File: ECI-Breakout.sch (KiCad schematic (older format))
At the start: 4 parts, among them P1 CONN_02X07

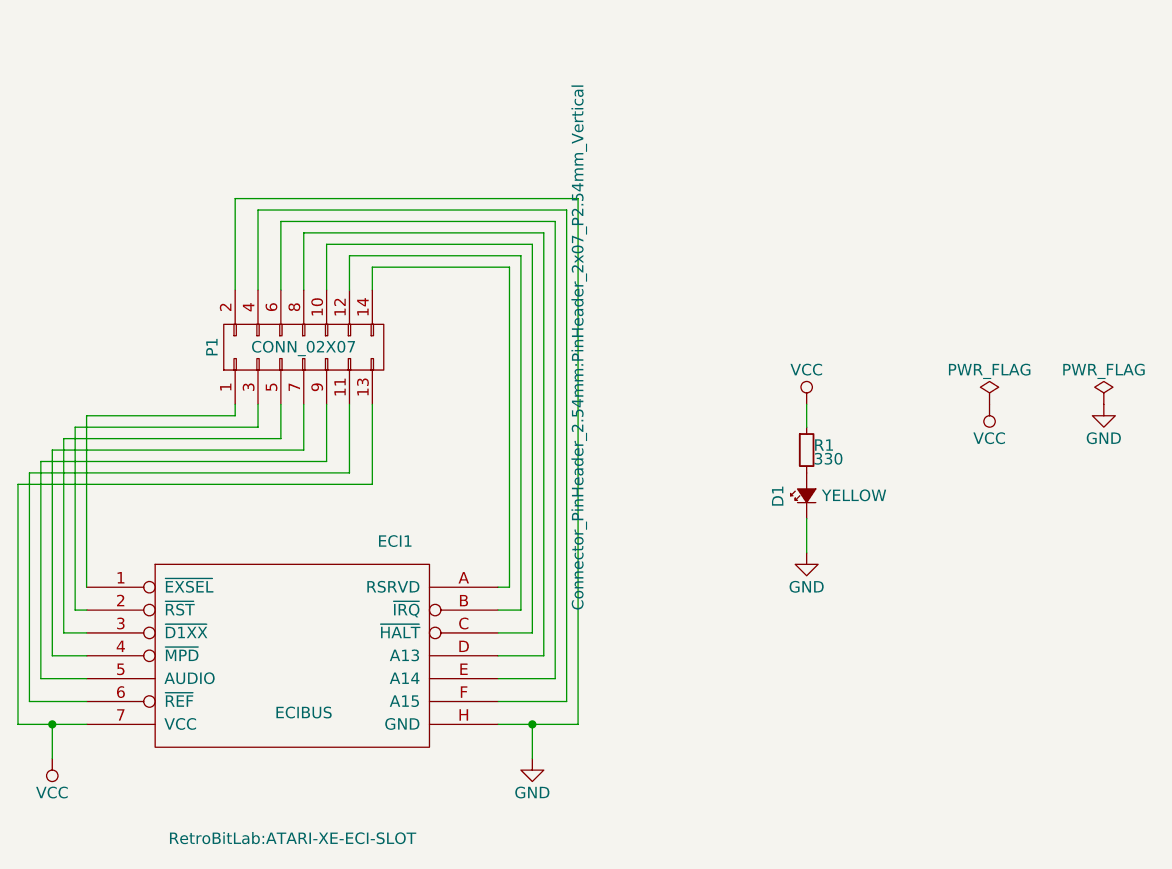
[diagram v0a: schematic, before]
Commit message: First elaborate project
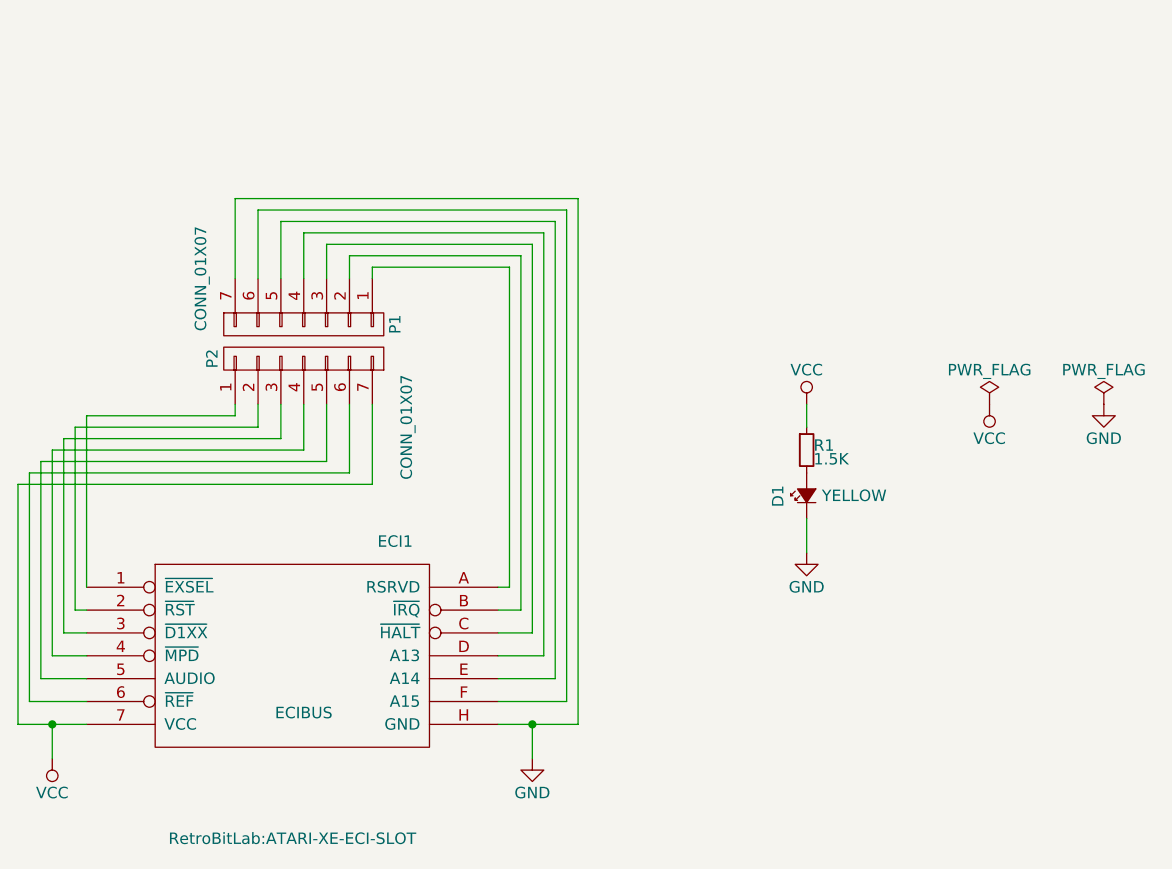
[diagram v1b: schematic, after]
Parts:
- removed P1: CONN_02X07, Connector_PinHeader_2.54mm:PinHeader_2x07_P2.54mm_Vertical, symbol CONN_02X07
- added P1, P2: CONN_01X07, Pin_Headers:Pin_Header_Straight_1x07, symbol CONN_01X07
- R1: value 330 -> 1.5K; footprint Resistors_SMD:R_1210_HandSoldering -> Resistors_SMD:R_1206_HandSoldering
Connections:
- net GND: now also P1.7 (P7)
- net VCC: now also P2.7 (P7)
- net at ECI1.1 (~EXSEL): now also P2.1 (P1)
- net at ECI1.2 (~RST): now also P2.2 (P2)
- net at ECI1.3 (~D1XX): now also P2.3 (P3)
- net at ECI1.4 (~MPD): now also P2.4 (P4)
- net at ECI1.5 (AUDIO): now also P2.5 (P5)
- net at ECI1.6 (~REF): now also P2.6 (P6)
- net at ECI1.A (RSRVD): now also P1.1 (P1)
- net at ECI1.B (~IRQ): now also P1.2 (P2)
- net at ECI1.C (~HALT): now also P1.3 (P3)
- net at ECI1.D (A13): now also P1.4 (P4)
- net at ECI1.E (A14): now also P1.5 (P5)
- net at ECI1.F (A15): now also P1.6 (P6)
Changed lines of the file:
@@
 P 7800 2850
 F 0 "R1" H 7830 2870 50  0000 L CNN
-F 1 "330" H 7830 2810 50  0000 L CNN
-F 2 "Resistors_SMD:R_1210_HandSoldering" H 7800 2850 50  0001 C CNN
+F 1 "1.5K" H 7830 2810 50  0000 L CNN
+F 2 "Resistors_SMD:R_1206_HandSoldering" H 7800 2850 50  0001 C CNN
 F 3 "" H 7800 2850 50  0000 C CNN
 	1    7800 2850
@@
 	1    0    0    -1
 $EndComp
-$Comp
-L CONN_02X07 P1
-U 1 1 5CADC0E2
-P 5600 2400
-F 0 "P1" H 5600 2800 50  0000 C CNN
-F 1 "CONN_02X07" V 5600 2400 50  0000 C CNN
-F 2 "Connector_PinHeader_2.54mm:PinHeader_2x07_P2.54mm_Vertical" H 5600 1200 50  0000 C CNN
-F 3 "" H 5600 1200 50  0000 C CNN
-	1    5600 2400
-	0    -1   -1   0
-$EndComp
 Wire Wire Line
 	4650 3450 4650 2700
@@
 Connection ~ 4500 4050
 Wire Wire Line
-	5900 2150 5900 2050
-Wire Wire Line
 	5900 2050 6500 2050
 Wire Wire Line
@@
 	6550 2000 5800 2000
 Wire Wire Line
-	5800 2000 5800 2150
-Wire Wire Line
 	6450 3650 6600 3650
 Wire Wire Line
@@
 	6600 1950 5700 1950
 Wire Wire Line
-	5700 1950 5700 2150
-Wire Wire Line
 	6450 3750 6650 3750
 Wire Wire Line
@@
 	6650 1900 5600 1900
 Wire Wire Line
-	5600 1900 5600 2150
-Wire Wire Line
 	6450 3850 6700 3850
 Wire Wire Line
@@
 	6700 1850 5500 1850
 Wire Wire Line
-	5500 1850 5500 2150
-Wire Wire Line
 	6450 3950 6750 3950
 Wire Wire Line
@@
 Wire Wire Line
 	6750 1800 5400 1800
-Wire Wire Line
-	5400 1800 5400 2150
-Wire Wire Line
-	5300 2150 5300 1750
 Wire Wire Line
 	5300 1750 6800 1750
@@
 	6800 1750 6800 4050
 Connection ~ 6600 4050
+$Comp
+L CONN_01X07 P1
+U 1 1 5CB38837
+P 5600 2300
+F 0 "P1" H 5600 2700 50  0000 C CNN
+F 1 "CONN_01X07" H 5400 1850 50  0000 C CNN
+F 2 "Pin_Headers:Pin_Header_Straight_1x07" H 5600 2300 50  0001 C CNN
+F 3 "" H 5600 2300 50  0000 C CNN
+	1    5600 2300
+	0    1    1    0
+$EndComp
+$Comp
+L CONN_01X07 P2
+U 1 1 5CB388A4
+P 5600 2450
+F 0 "P2" H 5600 2850 50  0000 C CNN
+F 1 "CONN_01X07" H 5300 2000 50  0000 C CNN
+F 2 "Pin_Headers:Pin_Header_Straight_1x07" H 5600 2450 50  0001 C CNN
+F 3 "" H 5600 2450 50  0000 C CNN
+	1    5600 2450
+	0    -1   -1   0
+$EndComp
+Wire Wire Line
+	5900 2050 5900 2100
+Wire Wire Line
+	5800 2000 5800 2100
+Wire Wire Line
+	5700 1950 5700 2100
+Wire Wire Line
+	5600 1900 5600 2100
+Wire Wire Line
+	5500 1850 5500 2100
+Wire Wire Line
+	5400 1800 5400 2100
+Wire Wire Line
+	5300 1750 5300 2100
 $EndSCHEMATC
